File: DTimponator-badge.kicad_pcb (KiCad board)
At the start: 2 copper layers, 96.5 x 96.5 mm, 42 parts, among them J1 AVR-ISP, SW1 SW_SPDT, SW2 SW_Push, U1 74HC595, U2 ATtiny85-20S, U3 74HC595

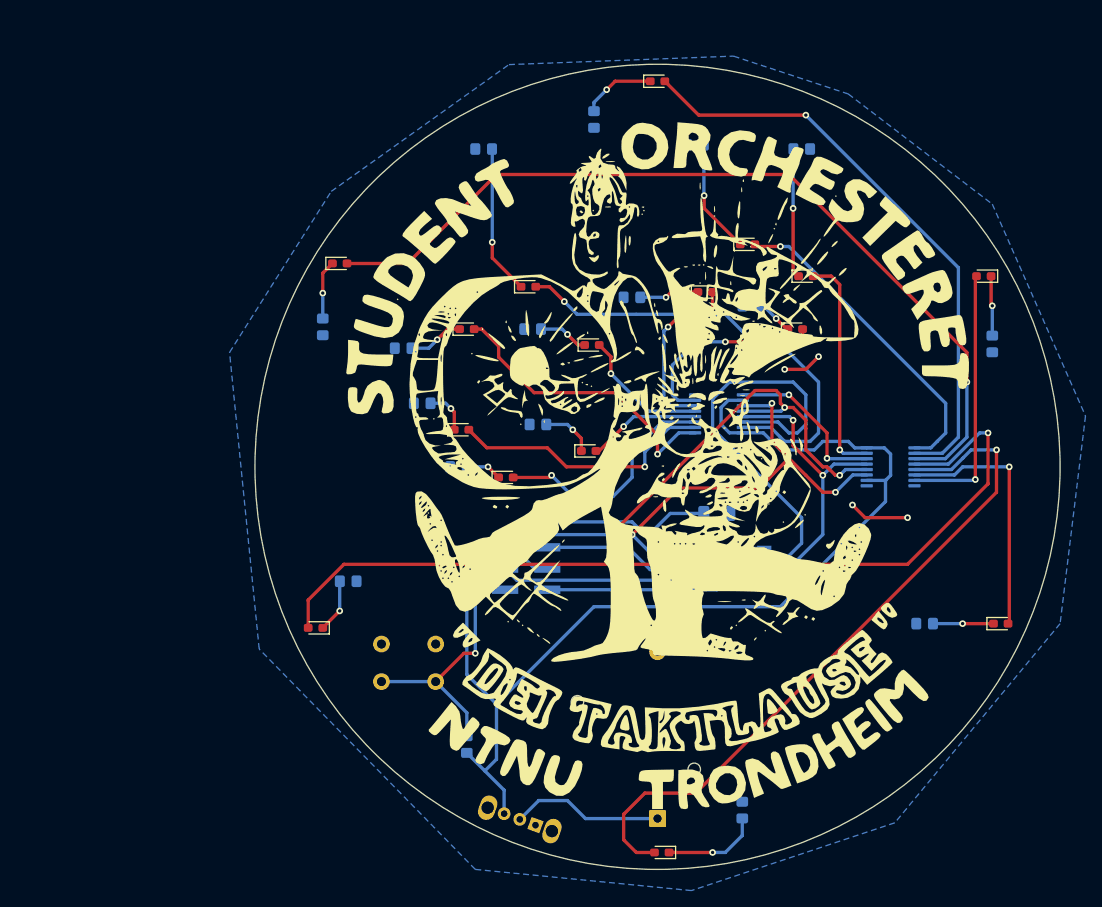
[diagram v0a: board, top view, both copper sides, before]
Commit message: Made V2
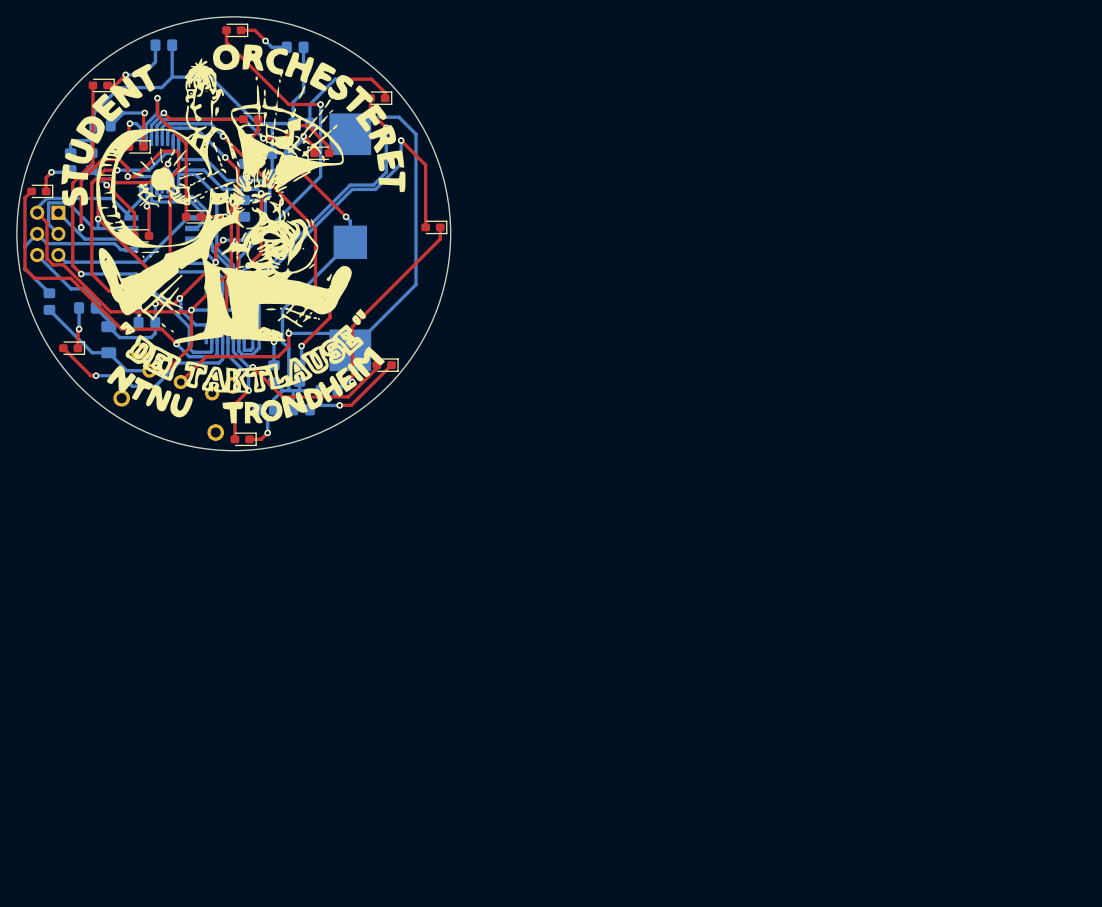
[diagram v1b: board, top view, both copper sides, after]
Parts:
- removed C1, 1uF: .1uF, Capacitor_SMD:C_1206_3216Metric_Pad1.33x1.80mm_HandSolder
- removed R9, 10k: 10k, Resistor_SMD:R_0805_2012Metric_Pad1.20x1.40mm_HandSolder
- removed SW2: SW_Push, Button_Switch_THT:SW_PUSH_6mm_H5mm
- added C1: .1uF, Capacitor_SMD:C_1206_3216Metric_Pad1.33x1.80mm_HandSolder, B.Cu at (89.2, 73.7)
- added R9: 10k, Resistor_SMD:R_0805_2012Metric_Pad1.20x1.40mm_HandSolder, B.Cu at (82.0, 69.1)
- BT1: footprint DTimponator-badge:MP000362_CR2032_Holder_THT -> Battery:BatteryHolder_Multicomp_BC-2001_1x2032
- J1: footprint Connector_PinHeader_2.54mm:PinHeader_2x03_P2.54mm_Vertical_SMD -> Connector_PinHeader_2.54mm:PinHeader_2x03_P2.54mm_Horizontal
- SW1: footprint DTimponator-badge:OS102011MA1QN1_SPDT_SlideSwithch_THT -> Button_Switch_THT:SW_E-Switch_EG1224_SPDT_Angled
- moved D15 126.4 mm to (80.8, 55.9), turned to 180 degrees
- moved R16 116.4 mm to (84.6, 52.3), turned to 90 degrees
- moved D16 108.4 mm to (88.1, 43.2)
- moved R17 105.6 mm to (95.8, 38.4), turned to 0 degrees
- moved R15 98.9 mm to (86.6, 69.8), turned to 0 degrees
- moved D14 93.1 mm to (84.6, 74.7)
- moved U3 81.8 mm to (103.1, 70.6), turned to 90 degrees
- moved D8 80.1 mm to (91.4, 67.8), turned to 180 degrees
- moved U2 79.2 mm to (95.5, 61.0)
- moved D9 74.6 mm to (104.1, 36.6), turned to 180 degrees
- moved U1 73.4 mm to (95.2, 52.6), turned to -90 degrees
- moved R8 72.4 mm to (93.7, 71.6), turned to 0 degrees
- moved J1 70.5 mm to (83.1, 58.4)
- moved BT1 66.3 mm to (118.1, 62.0), turned to 90 degrees
- moved SW1 63.0 mm to (101.5, 80.1)
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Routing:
- net GND: track 11.9 -> 178.2 mm, vias 4 -> 6
- net Net-(D13-A): track 107.1 -> 13.8 mm
- net Net-(D12-A): track 105.1 -> 22.9 mm
- net Net-(D14-A): track 84.0 -> 24.9 mm
- net Net-(D1-A): track 54.9 -> 5.92 mm
- net VCC: track 168.5 -> 122.3 mm, vias 0 -> 4
- net Net-(BT1-+): track 18.3 -> 63.2 mm, vias 0 -> 1
- net /SER: track 51.7 -> 10.9 mm
- net /MOSI: track 58.2 -> 21.1 mm, vias 1 -> 0
- net Net-(D2-A): track 35.9 -> 5.78 mm
- net /SCK: track 73.7 -> 52.0 mm
- net Net-(D11-A): track 70.8 -> 49.7 mm
- net Net-(D6-A): track 16.0 -> 33.5 mm
- net Net-(D11-K): track 8.85 -> 25.1 mm
- net /~{OE}_PWM: track 36.0 -> 20.2 mm, vias 2 -> 0
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- removed copper zone on B.Cu, net GND
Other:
- board size 96.5 x 96.5 mm -> 52 x 52 mm
